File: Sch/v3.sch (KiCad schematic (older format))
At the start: 32 parts

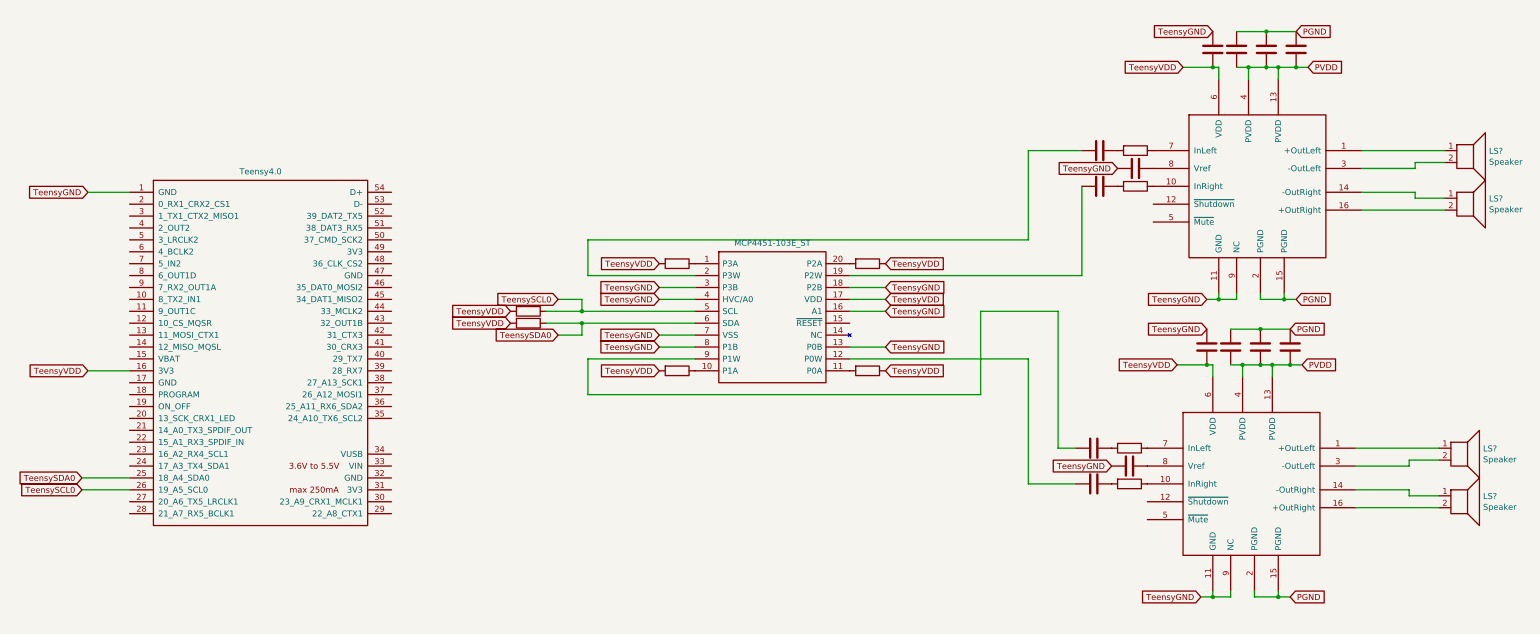
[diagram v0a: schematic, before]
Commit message: Small optimizations
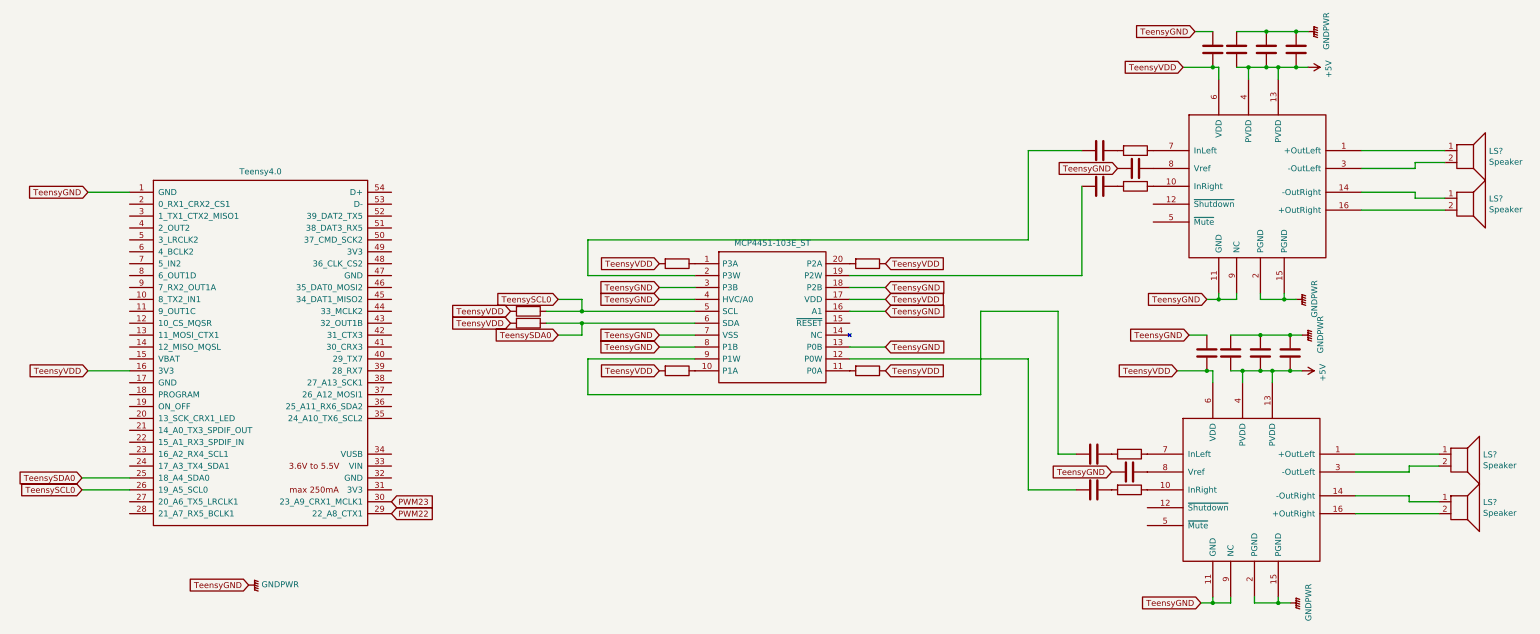
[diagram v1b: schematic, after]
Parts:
- removed C?: 0.1uF, symbol Device:C
- removed C? (x2): 0.47uF, symbol Device:C
- removed C? (x3): 1uF, symbol Device:C
- removed C?: 470uF, symbol Device:C
- removed LS? (x2): Speaker, symbol Device:Speaker
- removed R? (x2): 10000, symbol Device:R
- removed U?: PAM8403, symbol pam8403:PAM8403
- added C?: 0.1uF, symbol Device:C
- added C? (x2): 0.47uF, symbol Device:C
- added C? (x3): 1uF, symbol Device:C
- added C?: 470uF, symbol Device:C
- added LS? (x2): Speaker, symbol Device:Speaker
- added R? (x2): 10000, symbol Device:R
- added U?: PAM8403, symbol pam8403:PAM8403
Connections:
- net TeensyGND is gone; now on net GNDPWR: C?.1, C?.2, IC?.13 (P0B), IC?.16 (A1), IC?.18 (P2B), IC?.3 (P3B), IC?.4 (HVC/A0), IC?.7 (VSS), IC?.8 (P1B), U?.1 (GND), U?.11 (GND), U?.9 (NC)
- net TeensyVDD: now also C?.2, U?.6 (VDD)
- net PWM22: now reaches U?.29 (22_A8_CTX1)
- net PWM23: now reaches U?.30 (23_A9_CRX1_MCLK1)
- net at IC?.12 (P0W): now also C?.2
- net at IC?.9 (P1W): now also C?.2
- net PGND renamed GNDPWR
- net GNDPWR: now also C?.1, C?.1, C?.1, C?.1, C?.2, U?.11 (GND), U?.15 (PGND), U?.2 (PGND), U?.9 (NC)
- net PVDD renamed +5V
- net +5V: now also C?.2, C?.2, C?.2, U?.13 (PVDD), U?.4 (PVDD)
- new net: LS?.1, U?.1 (+OutLeft)
- new net: R?.1, U?.10 (InRight)
- new net: LS?.1, U?.14 (-OutRight)
- new net: LS?.2, U?.16 (+OutRight)
- new net: LS?.2, U?.3 (-OutLeft)
- new net: R?.1, U?.7 (InLeft)
- new net: C?.1, U?.8 (Vref)
- new net: C?.1, R?.2 (x2)
